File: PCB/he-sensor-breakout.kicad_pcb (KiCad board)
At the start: 2 copper layers, 95.3 x 86.8 mm, 160 parts, among them J1 Conn_01x03, U1 SLSS49E

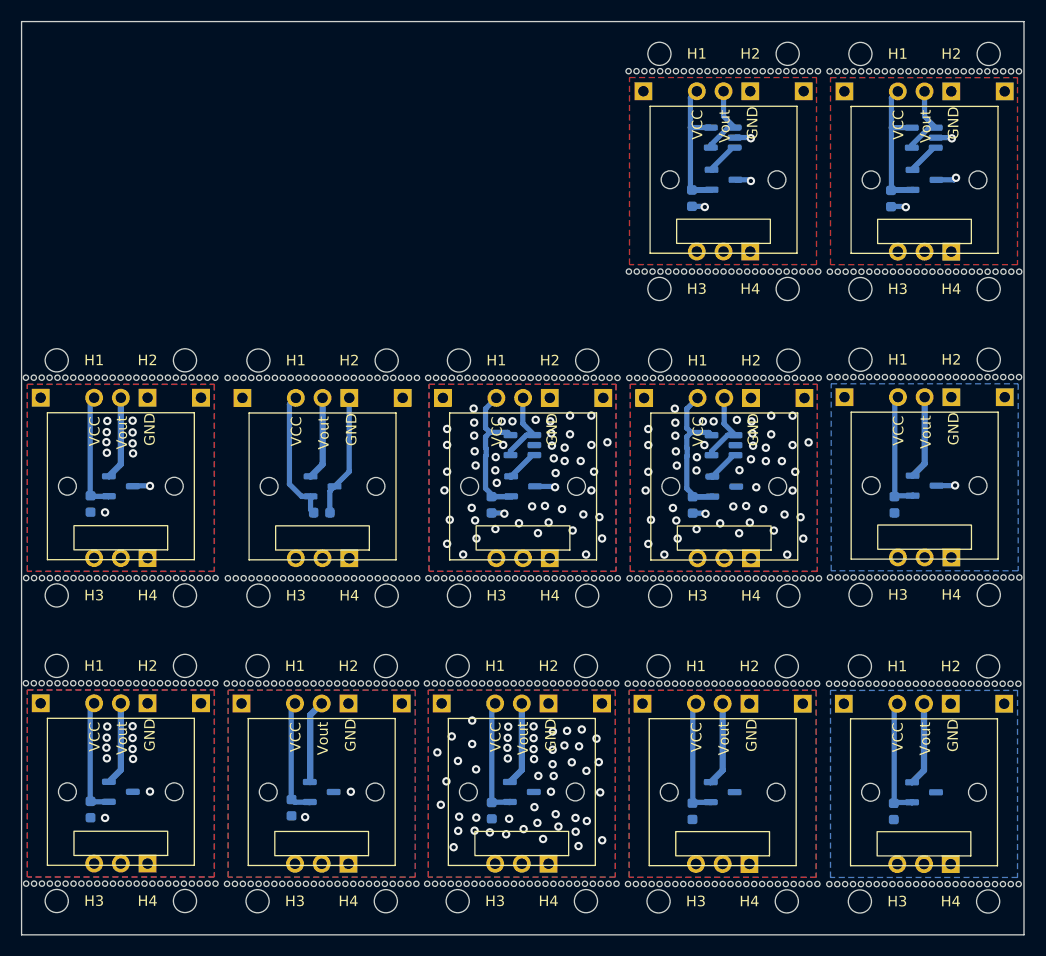
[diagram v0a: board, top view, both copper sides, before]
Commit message: adds tb
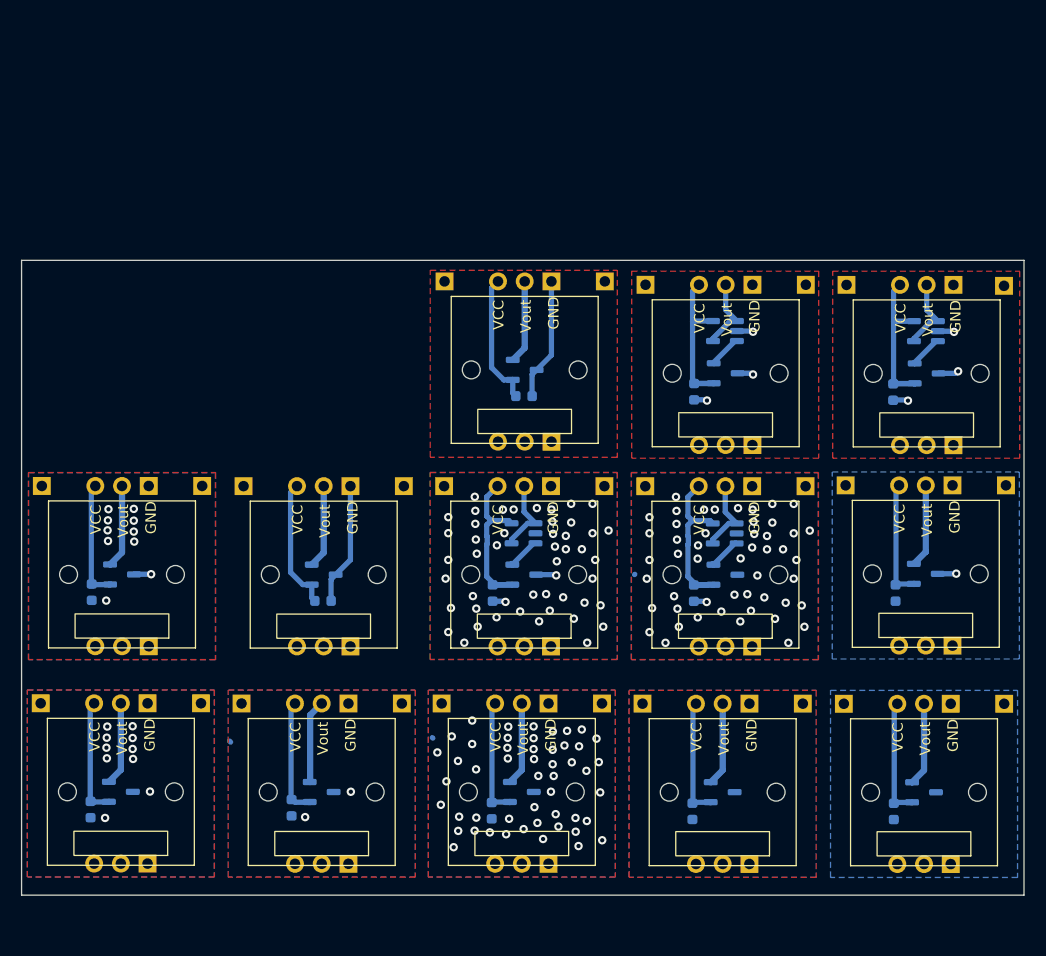
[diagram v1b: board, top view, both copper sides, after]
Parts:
- removed H1 (x12), H2 (x12), H3 (x12), H4 (x12): MountingHole_2.2mm_M2, MountingHole:MountingHole_2.2mm_M2
- removed MOUSE1 (x12), MOUSE2 (x12): mouse-bite-19mm, Panelization:mouse-bite-19mm
- removed REF** (x3): SOT-23-5, Package_TO_SOT_SMD:SOT-23-5
- added C1: 100n, Capacitor_SMD:C_0603_1608Metric, B.Cu at (119.2, 59.2)
- added J1: Conn_01x03, Connector_PinHeader_2.54mm:PinHeader_1x03_P2.54mm_Vertical, B.Cu at (121.8, 48.3)
- added STB1: PinHeader_1x01_P2.54mm_Vertical, Connector_PinHeader_2.54mm:PinHeader_1x01_P2.54mm_Vertical, B.Cu at (111.7, 48.3)
- added STB2: PinHeader_1x01_P2.54mm_Vertical, Connector_PinHeader_2.54mm:PinHeader_1x01_P2.54mm_Vertical, B.Cu at (126.9, 48.3)
- added STB3: PinHeader_1x03_P2.54mm_Vertical, Connector_PinHeader_2.54mm:PinHeader_1x03_P2.54mm_Vertical, B.Cu at (121.8, 63.5)
- added SW: SW_Lekker_MX_1.00u_PCB, Button_Switch_Keyboard:SW_Lekker_MX_1.00u_PCB, F.Cu at (119.3, 56.7)
- added U1: SLSS49E, Package_TO_SOT_SMD:SOT-23-3, B.Cu at (119.3, 56.7)
- added U3: MCP6001, Package_TO_SOT_SMD:SOT-23-5, B.Cu at (138.3, 53.0)
- added U3: MCP6001, Package_TO_SOT_SMD:SOT-23-5, B.Cu at (119.2, 72.2)
- added U3: MCP6001, Package_TO_SOT_SMD:SOT-23-5, B.Cu at (138.3, 72.2)
- U3: renamed from REF**; value SOT-23-5 -> MCP6001
- moved STB2 18.5 mm to (164.9, 48.7)
- moved SW 18.4 mm to (138.4, 57.0)
- moved U1 18.4 mm to (138.4, 57.0)
- moved J1 18.4 mm to (141.0, 48.6)
- moved STB1 18.4 mm to (130.8, 48.6)
- moved STB2 18.4 mm to (146.0, 48.6)
- moved C1 18.4 mm to (154.3, 58.8)
- moved C1 18.4 mm to (135.4, 58.7)
- moved J1 18.4 mm to (160.1, 48.6)
- moved STB1 18.4 mm to (149.9, 48.6)
- moved STB3 18.4 mm to (141.0, 63.8)
- moved STB3 18.4 mm to (160.1, 63.8)
- moved SW 18.4 mm to (157.5, 57.0)
- moved U1 18.4 mm to (157.5, 57.0)
- moved U3 18.4 mm to (157.4, 53.0)
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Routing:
- net VCC: track 151.0 -> 163.6 mm
- net GND: track 28.6 -> 40.5 mm, vias 180 -> 178
- net /Vout: track 92.4 -> 100.4 mm
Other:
- board size 95.3 x 86.8 mm -> 95.3 x 60.3 mm
